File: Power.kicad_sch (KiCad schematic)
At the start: 27 parts, among them U1 LMR14030SDDAR, U5 TPS560430

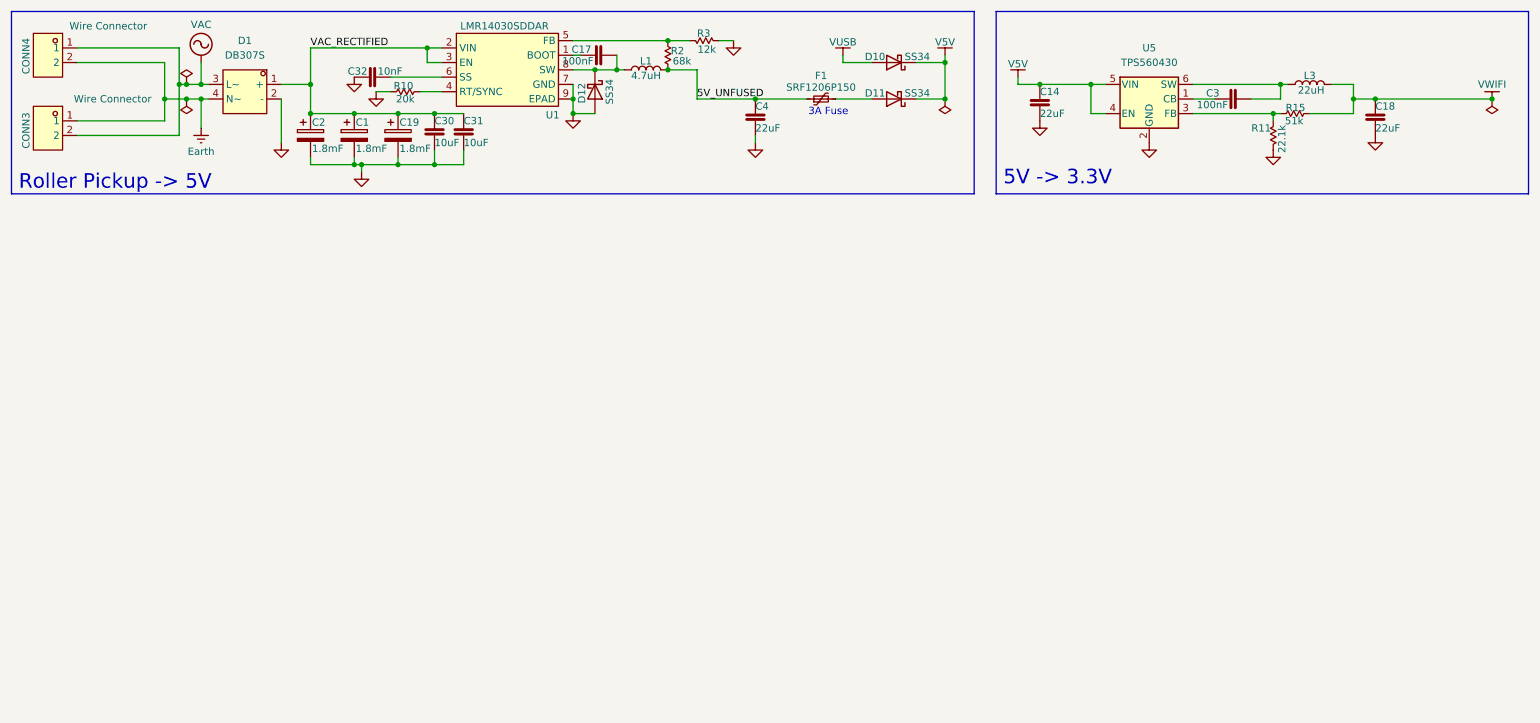
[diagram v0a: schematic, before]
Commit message: release evt2
Signed-off-by: Sean Cross <sean@xobs.io>
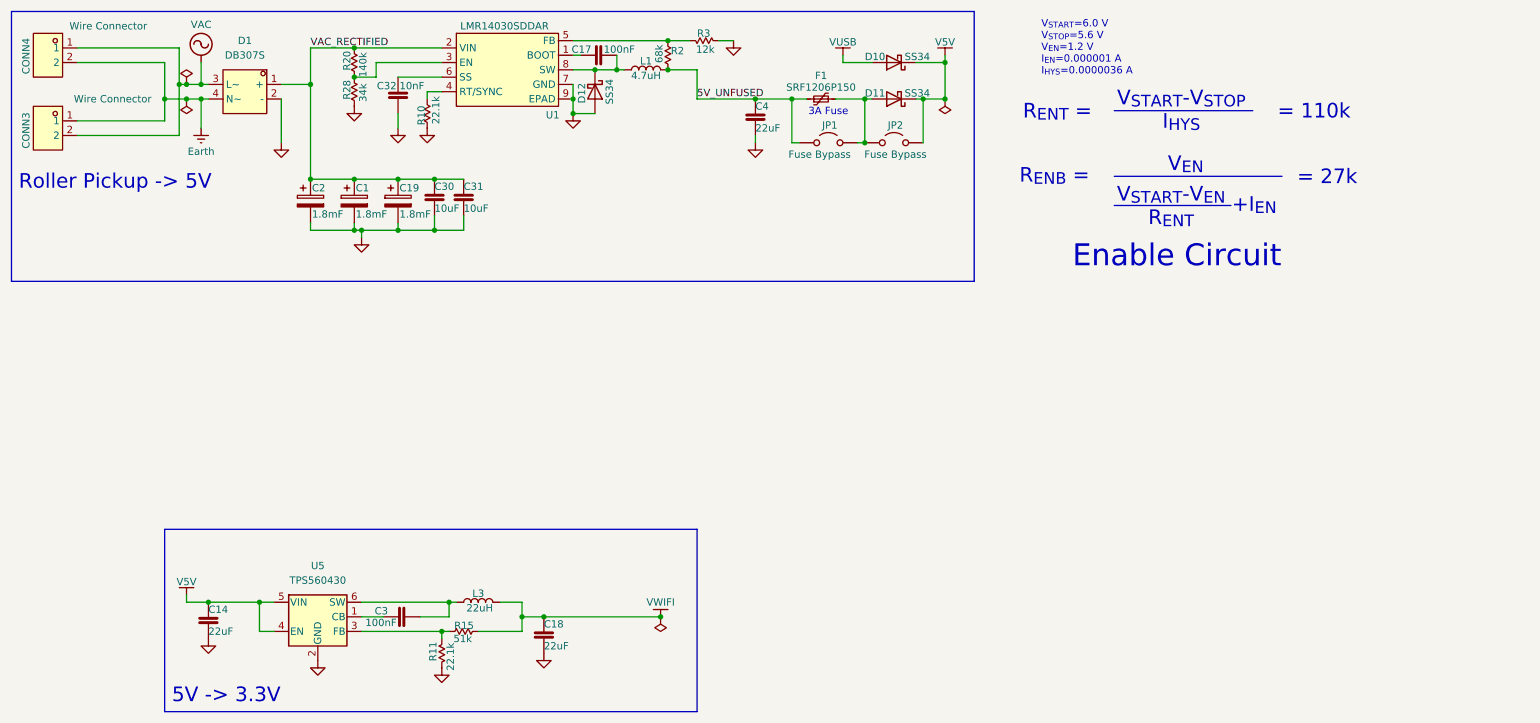
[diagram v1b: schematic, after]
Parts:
- added JP1, JP2: Fuse Bypass, Jumper:SolderJumper-2_P1.3mm_Open_TrianglePad1.0x1.5mm, symbol Jumper:Jumper_2_Open
- added R20: R 140k 0201, Galvani:R_0201_0603Metric, symbol Galvani:R 140k 0201
- added R28: R 34k 0201, Galvani:R_0201_0603Metric, symbol Galvani:R 34k 0201
- R10: value R 20k 0201 -> R 22.1k 0201; symbol Galvani:R 20k 0201 -> Galvani:R 22.1k 0201; Val 20k -> 22.1k
- R2: value R 68k 0402 -> R 68k 0201; footprint Resistor_SMD:R_0402_1005Metric -> Galvani:R_0201_0603Metric; symbol Galvani:R 68k 0402 -> Galvani:R 68k 0201
- R3: value R 12k 0402 -> R 12k 0201; footprint Resistor_SMD:R_0402_1005Metric -> Galvani:R_0201_0603Metric; symbol Galvani:R 12k 0402 -> Galvani:R 12k 0201
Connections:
- net 5V_UNFUSED: now also JP1.1 (A)
- net GND: now also R28.2
- net V5V: now also JP2.2 (B)
- net VAC_RECTIFIED: now also R20.1; no longer U1.3 (EN)
- net at D11.2 (A), F1.2: now also JP1.2 (B), JP2.1 (A)
- new net: R20.2, R28.1, U1.3 (EN)
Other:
- note added: "+I_{EN}"
- note added: "= 110k"
- note added: "= 27k"
- note added: "Enable Circuit"
- note added: "R_{ENB} ="
- note added: "R_{ENT} ="
- note added: "V_{EN}"
- note added: "V_{START}-V_{EN} R_{ENT}"
- note added: "V_{START}-V_{STOP} I_{HYS}"
- note added: "V_{START}=6.0 V V_{STOP}=5.6 V V_{EN}=1.2 V I_{EN}=0.000001 A I_{HYS}=0.0000036 A"
- moved on the sheet: C1, C14, C18, C19, C2, C3, C30, C31, C32, L3, R10, R11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
